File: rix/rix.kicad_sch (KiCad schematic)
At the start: 13 parts, among them J1 Barrel_Jack_Switch, J2 Conn_01x02_Male, J3 Conn_01x01_Male, U1 74LS04, U2 L78L05_SOT89, Y1 Crystal, Y2 Crystal

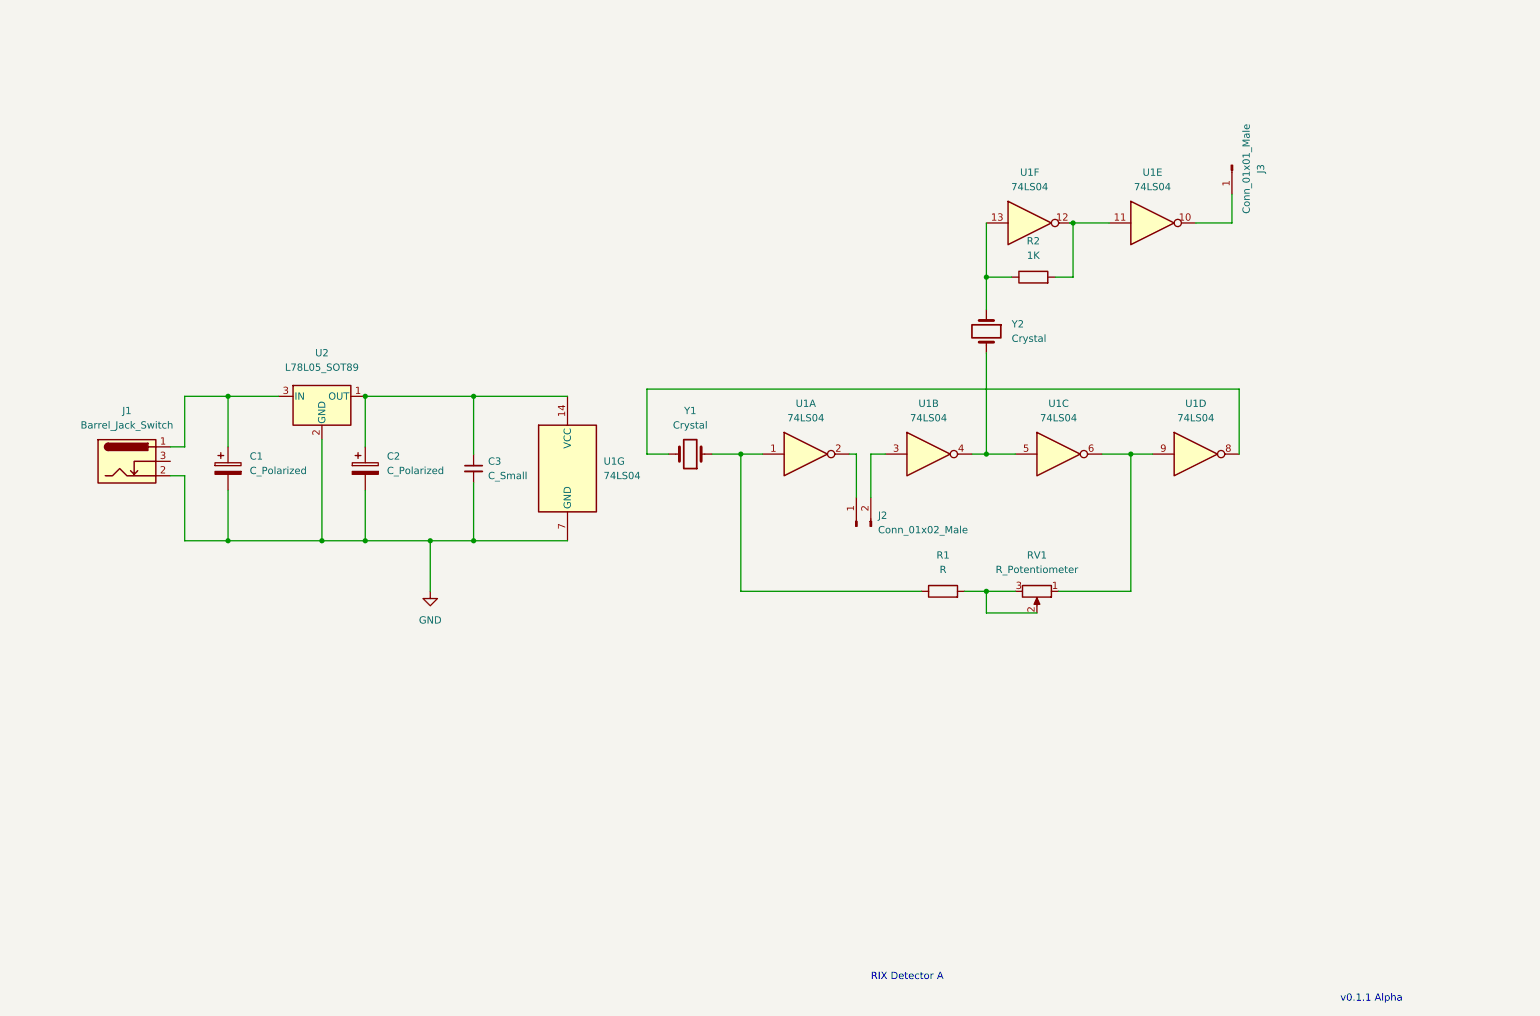
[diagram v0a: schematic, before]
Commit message: PCB improvements
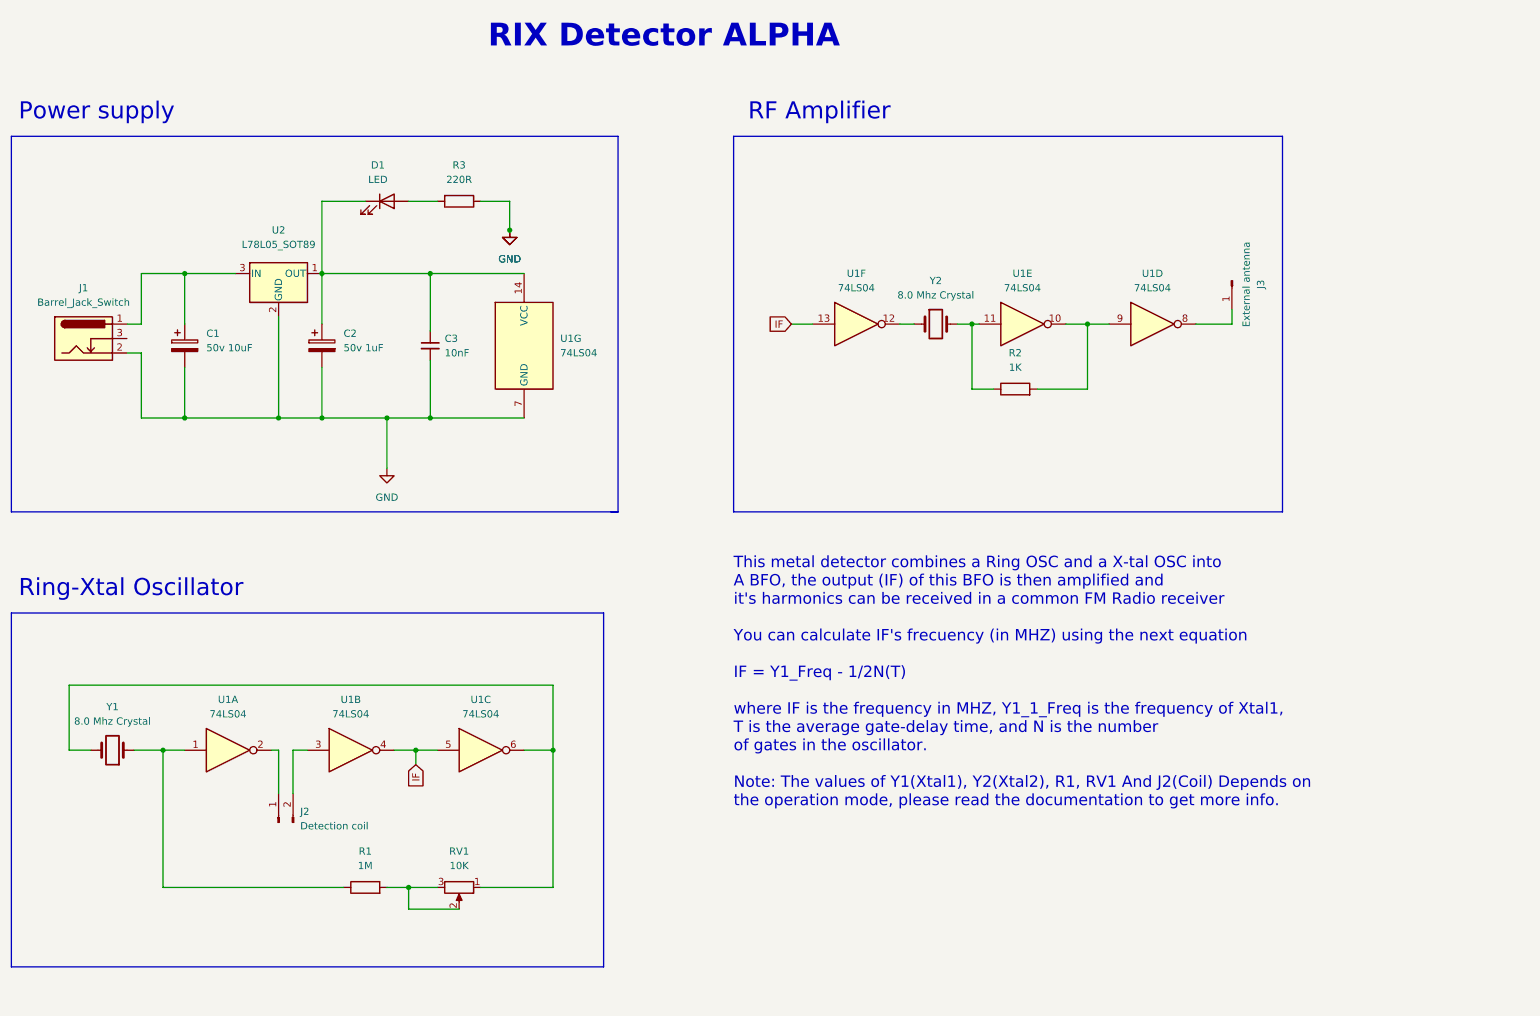
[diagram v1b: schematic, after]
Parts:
- added D1: LED, Diode_SMD:D_1206_3216Metric_Pad1.42x1.75mm_HandSolder, symbol Device:LED
- added R3: 220R, Resistor_SMD:R_0805_2012Metric_Pad1.20x1.40mm_HandSolder, symbol Device:R
- C1: value C_Polarized -> 50v 10uF; footprint Capacitor_THT:CP_Radial_D8.0mm_P3.50mm -> Capacitor_THT:CP_Radial_D5.0mm_P2.00mm
- C2: value C_Polarized -> 50v 1uF; footprint Capacitor_THT:CP_Radial_D8.0mm_P3.80mm -> Capacitor_THT:CP_Radial_D5.0mm_P2.00mm
- C3: value C_Small -> 10nF; footprint Capacitor_SMD:C_1206_3216Metric_Pad1.33x1.80mm_HandSolder -> Capacitor_SMD:C_0805_2012Metric_Pad1.18x1.45mm_HandSolder
- J1: footprint Connector_BarrelJack:BarrelJack_Horizontal -> Connector_BarrelJack:BarrelJack_Kycon_KLDX-0202-xC_Horizontal
- J2: value Conn_01x02_Male -> Detection coil; footprint Connector_PinSocket_2.54mm:PinSocket_1x02_P2.54mm_Vertical -> Connector_PinHeader_2.54mm:PinHeader_1x02_P2.54mm_Vertical
- J3: value Conn_01x01_Male -> External antenna; footprint Connector_Pin:Pin_D1.4mm_L8.5mm_W2.8mm_FlatFork -> Connector_PinHeader_2.54mm:PinHeader_1x01_P2.54mm_Vertical
- R1: value R -> 1M
- RV1: value R_Potentiometer -> 10K
- U1: footprint Package_SO:SO-14_3.9x8.65mm_P1.27mm -> Package_SO:SOIC-14_3.9x8.7mm_P1.27mm
- Y1, Y2: value Crystal -> 8.0 Mhz Crystal
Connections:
- net GND: now also R3.1
- net at C2.1, C3.1, U1.14 (VCC)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: now also D1.1 (K)
- net IF: now reaches U1.4, U1.5
- net IF: now also U1.13; no longer Y2.2
- net at RV1.1, U1.6: now also Y1.2; no longer U1.9
- net at U1.10: now also R2.2, U1.9; no longer J3.1 (Pin_1)
- net at U1.8: now also J3.1 (Pin_1); no longer Y1.2
- new net: U1.12, Y2.1
- new net: D1.2 (A), R3.2
- new net: R2.1, U1.11, Y2.2
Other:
- note added: "Power supply"
- note added: "RF Amplifier"
- note added: "RIX Detector ALPHA"
- note added: "Ring-Xtal Oscillator"
- note added: "This metal detector combines a Ring OSC and a X-tal OSC into A BFO, the output (IF) of this BFO is then amplified and it's harmonics can be received in a common FM Radio receiver You can calculate IF's frecuency (in MHZ) using the next equation IF = Y1_Freq - 1/2N(T) where IF is the frequency in MHZ, Y1_1_Freq is the frequency of Xtal1, T is the average gate-delay time, and N is the number of gat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"
- note removed: "RIX Detector A"
- note removed: "v0.1.1 Alpha"
- title: (none) -> RIX Metal Detector by Dionys.
- moved on the sheet: C1, C2, C3, J1, J2, J3, R1, R2, RV1, U1A, U1B, U1C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
